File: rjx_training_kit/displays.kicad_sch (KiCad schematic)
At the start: 30 parts, among them Q1 BC817, Q2 BC808, Q3 BC808, Q4 BC808, Q5 BC808, Q6 BC808, U4 LTC-4627JD (Red)

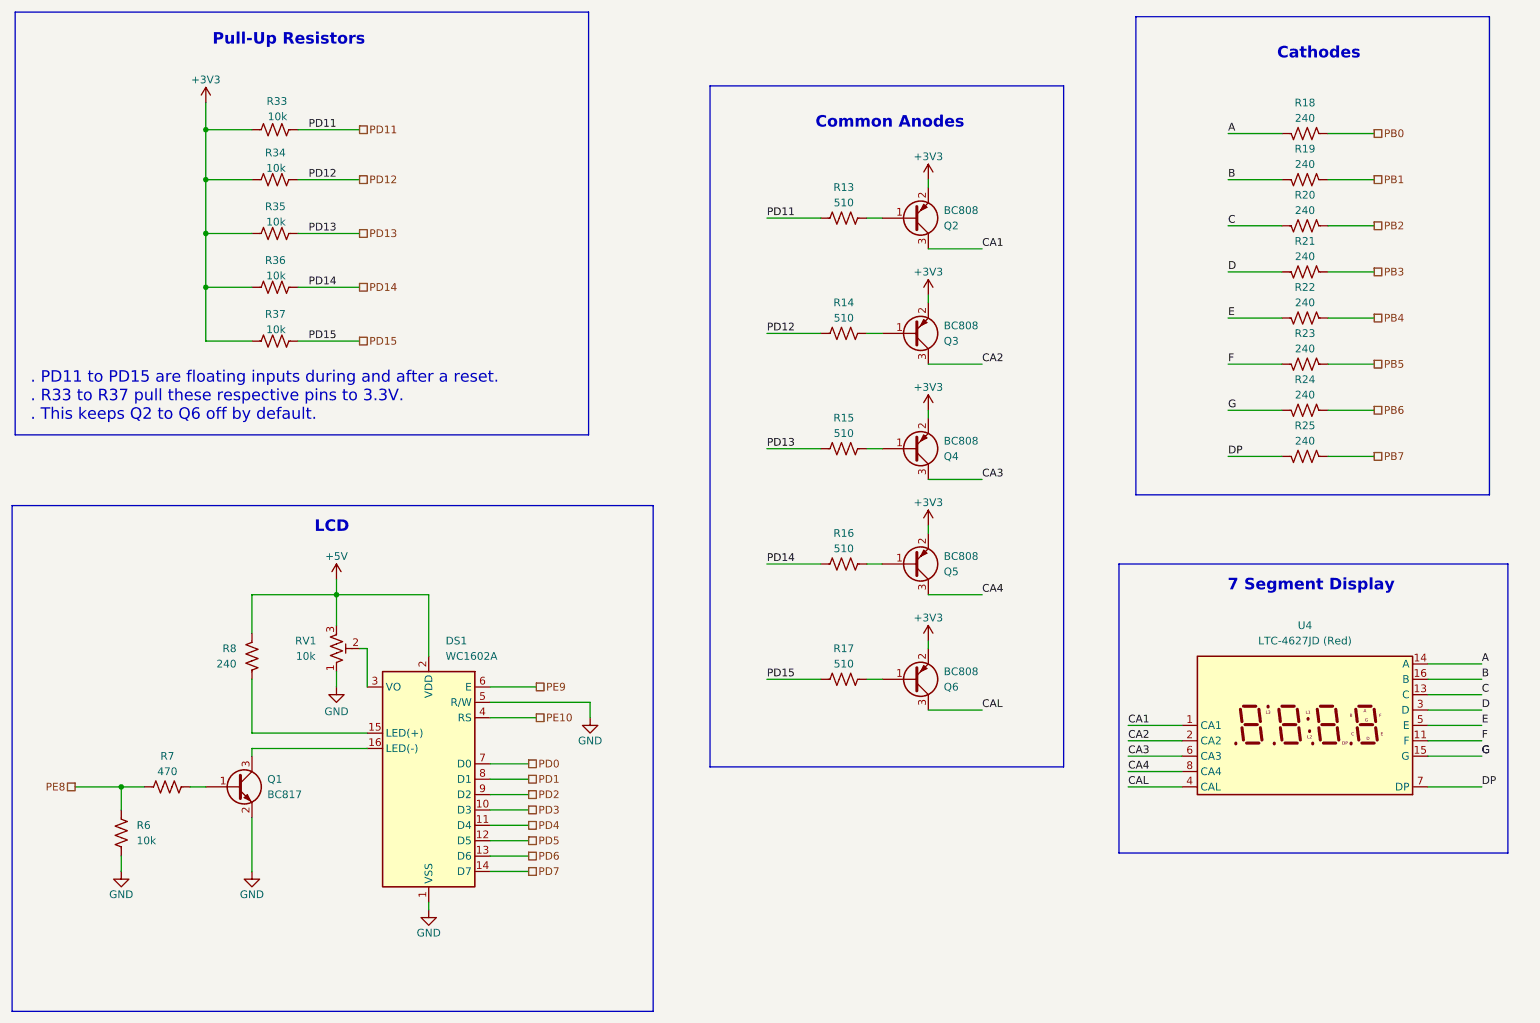
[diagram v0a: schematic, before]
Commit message: Update
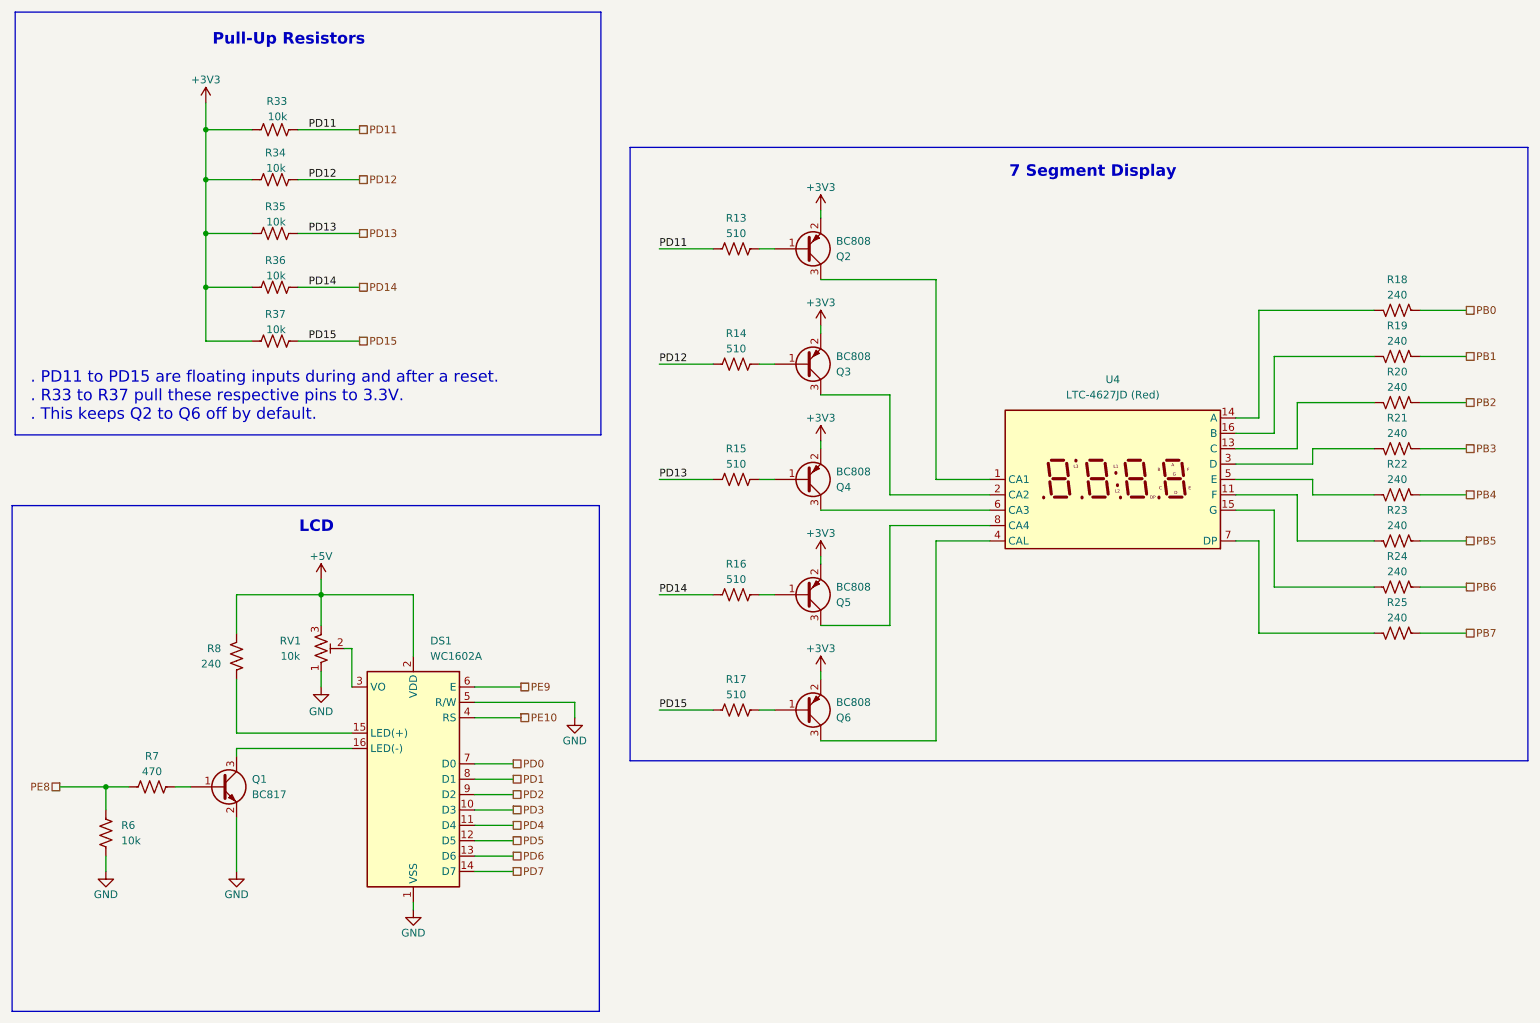
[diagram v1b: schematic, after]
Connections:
- net A: no longer names the net of R18.2, U4.14 (A)
- net B: no longer names the net of R19.2, U4.16 (B)
- net C: no longer names the net of R20.2, U4.13 (C)
- net CA1: no longer names the net of Q2.3 (C), U4.1 (CA1)
- net CA2: no longer names the net of Q3.3 (C), U4.2 (CA2)
- net CA3: no longer names the net of Q4.3 (C), U4.6 (CA3)
- net CA4: no longer names the net of Q5.3 (C), U4.8 (CA4)
- net CAL: no longer names the net of Q6.3 (C), U4.4 (CAL)
- net D: no longer names the net of R21.2, U4.3 (D)
- net DP: no longer names the net of R25.2, U4.7 (DP)
- net E: no longer names the net of R22.2, U4.5 (E)
- net F: no longer names the net of R23.2, U4.11 (F)
- net G: no longer names the net of R24.2, U4.15 (G)
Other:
- note removed: "Cathodes"
- note removed: "Common Anodes"
- moved on the sheet: DS1, Q1, Q2, Q3, Q4, Q5, Q6, R13, R14, R15, R16, R17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
